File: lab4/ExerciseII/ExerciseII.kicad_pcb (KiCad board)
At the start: 2 copper layers, 10 parts, among them J1 Conn_01x02_Male, U1 NE555D

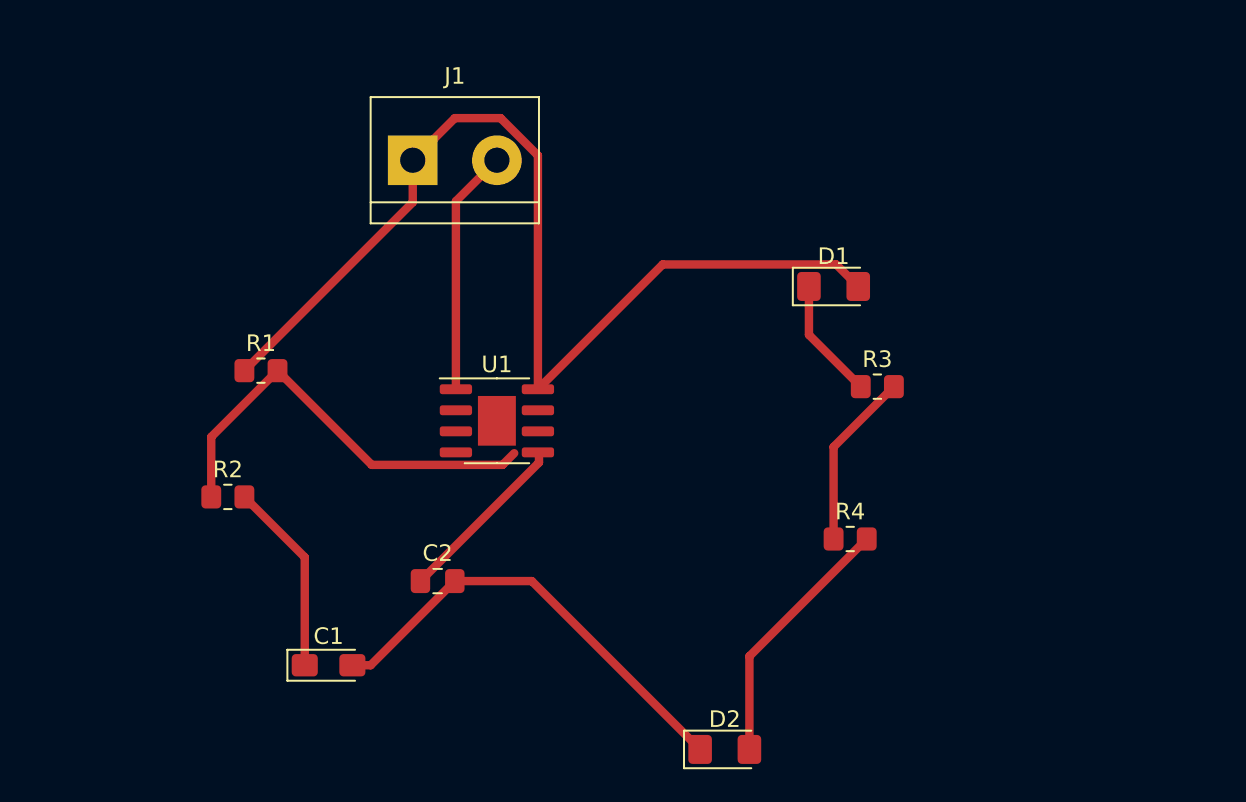
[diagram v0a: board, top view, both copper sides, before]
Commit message: ok
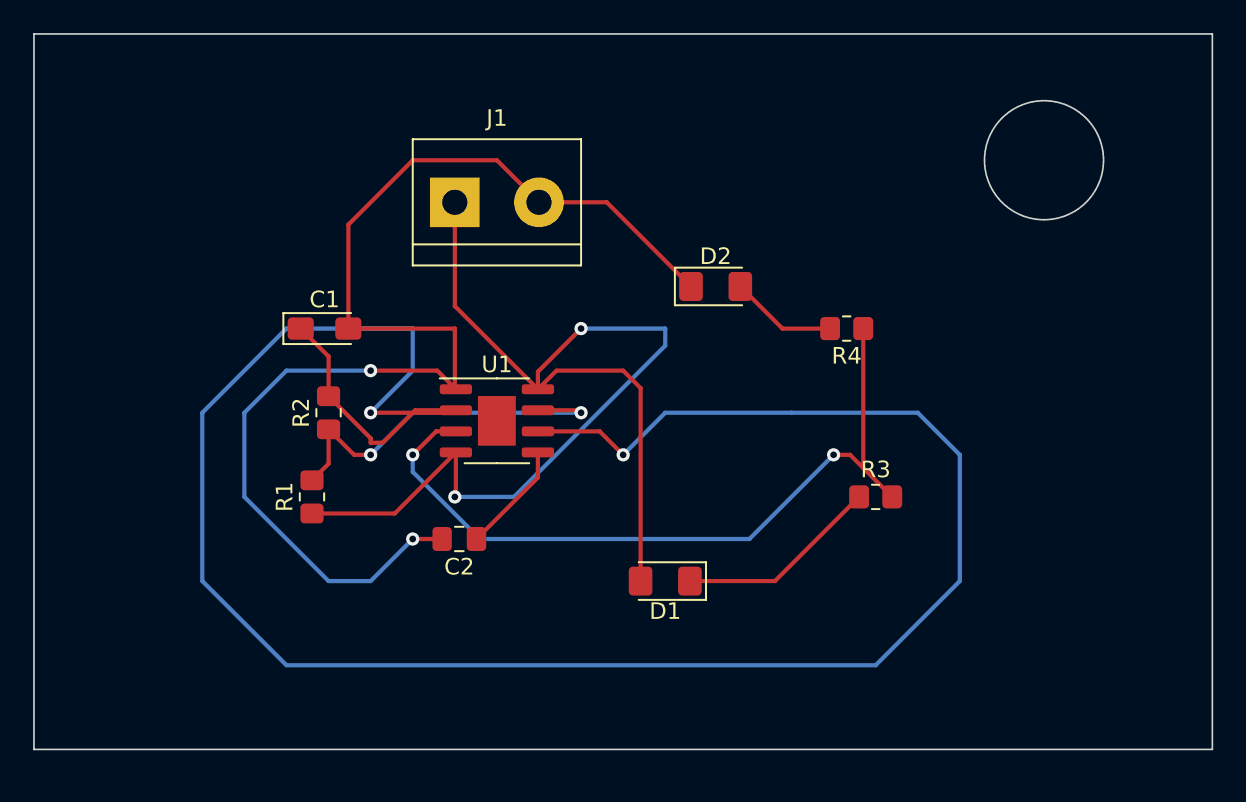
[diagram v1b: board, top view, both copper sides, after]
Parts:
- moved D2 27.9 mm to (155.4, 73.7)
- moved D1 20.5 mm to (152.4, 91.4), turned to 180 degrees
- moved C1 20.3 mm to (131.8, 76.2)
- moved R4 12.7 mm to (163.3, 76.2), turned to 180 degrees
- moved R1 8.22 mm to (131.1, 86.4), turned to 90 degrees
- moved R2 7.92 mm to (132.1, 81.3), turned to 90 degrees
- moved R3 6.66 mm to (165.1, 86.4)
- moved J1 3.59 mm to (139.7, 68.6)
- moved C2 2.86 mm to (140.0, 88.9), turned to 180 degrees
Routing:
- net /pin_2: track 12.0 -> 136.6 mm, vias 0 -> 2
- net /pin_3: track 10.7 -> 46.4 mm, vias 0 -> 2
- net GND: track 42.1 -> 76.3 mm, vias 0 -> 2
- net Net-(D2-Pad2): track 15.6 -> 6.47 mm
- net +9V: track 63.6 -> 72.4 mm, vias 0 -> 2
- net Net-(D1-Pad1): track 7.34 -> 12.3 mm
- net Net-(C2-Pad1): track 10.6 -> 6.76 mm
- net /pin_7: track 26.2 -> 23.1 mm, vias 0 -> 2
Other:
- board outline added: 71.1 x 43.2 mm
